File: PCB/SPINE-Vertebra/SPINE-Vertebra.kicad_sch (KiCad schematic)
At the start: 72 parts, among them J2 Conn_01x06, J4 Conn_01x06, J6 POWER, Q1 NTMFS5C628NLT1G, Q2 NTMFS5C628NLT1G, Q3 NTMFS5C628NLT1G, Q4 NTMFS5C628NLT1G, Q7 VISHAY SI2309CDS-T1-GE3, Q8 Q_NMOS_GSD, U1 ACS724xLCTR-50AB, U2 LM74800QDRRRQ1, U3 SP3485EN, U4 MIC5219-3.3YM5, U5 STM32G030F6Px

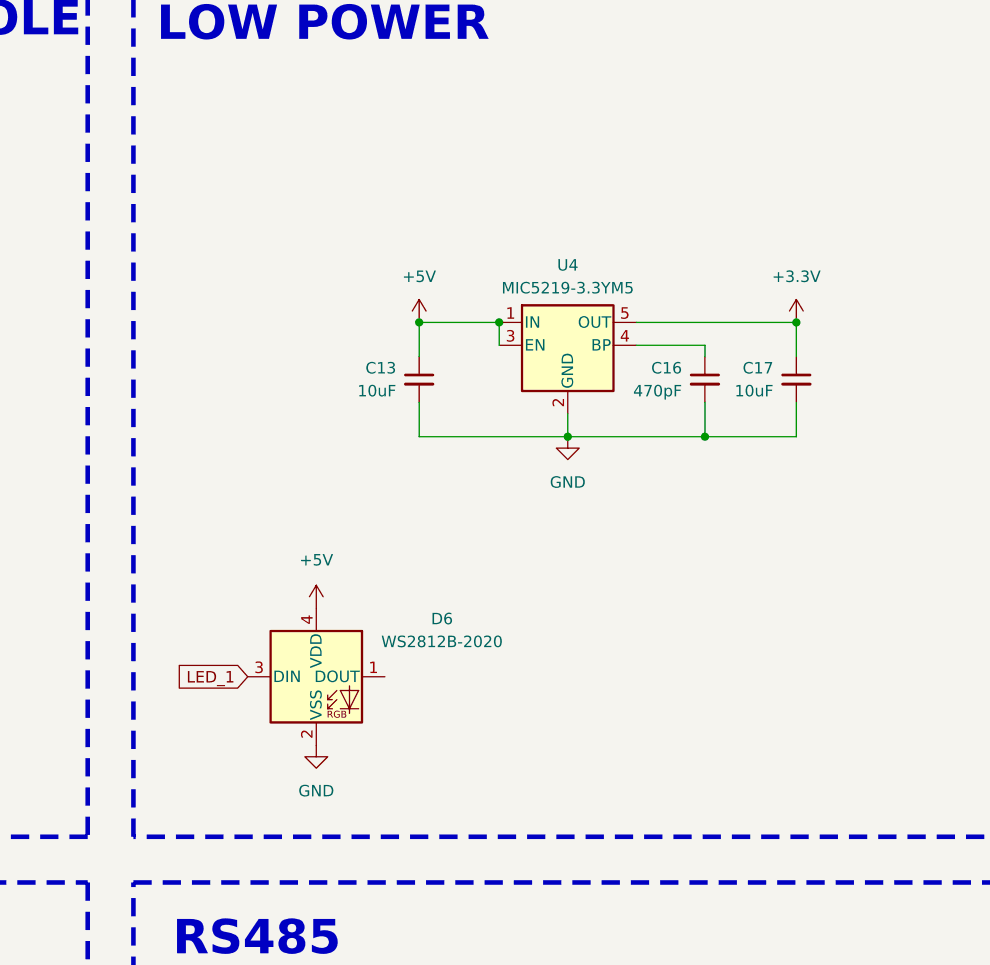
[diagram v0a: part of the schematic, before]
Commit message: update
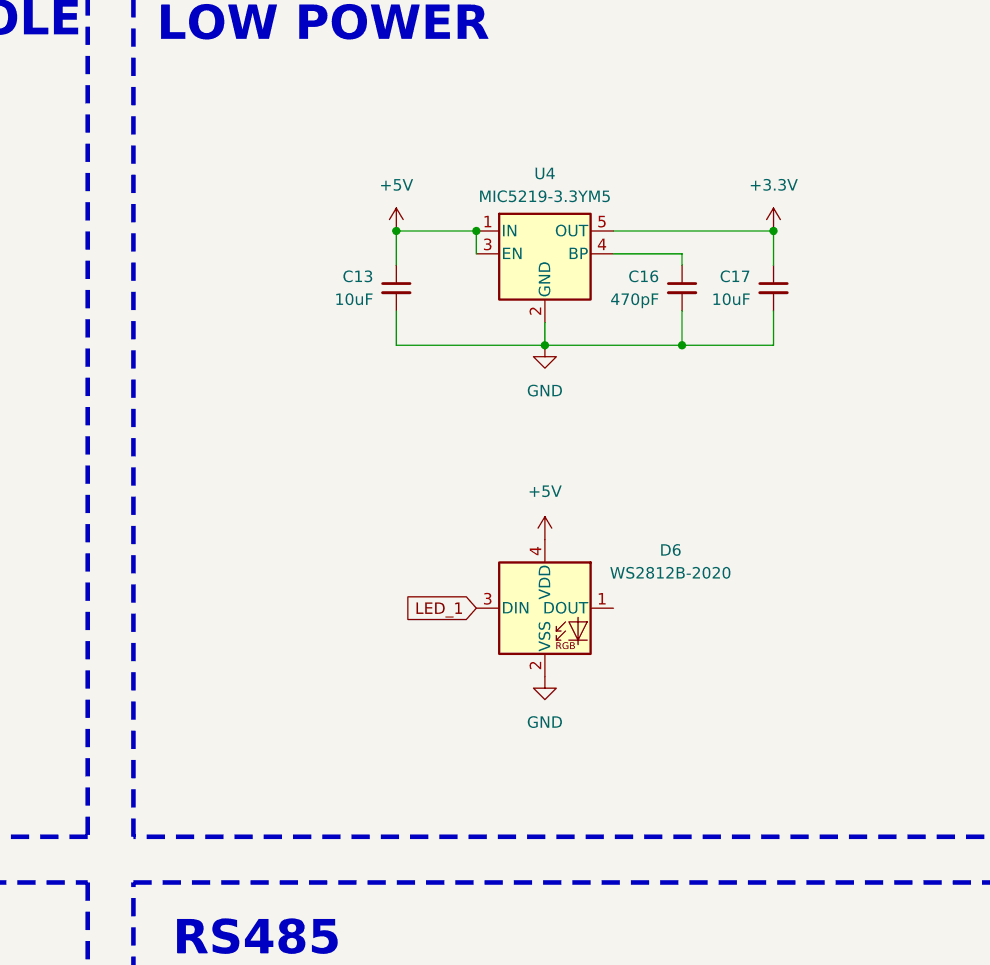
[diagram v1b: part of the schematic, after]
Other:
- moved on the sheet: C13, C16, C17, D6, U4
